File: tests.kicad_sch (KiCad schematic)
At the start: 11 parts, among them J101 USB_A+C+XT30

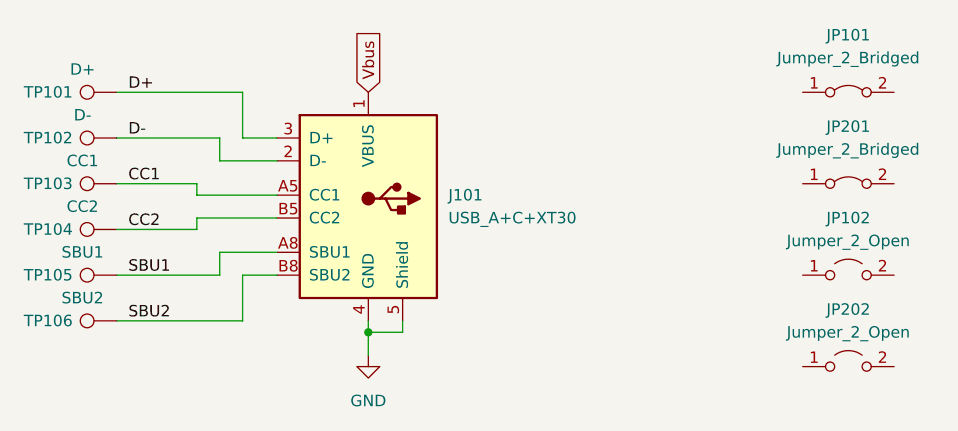
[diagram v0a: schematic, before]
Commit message: ...
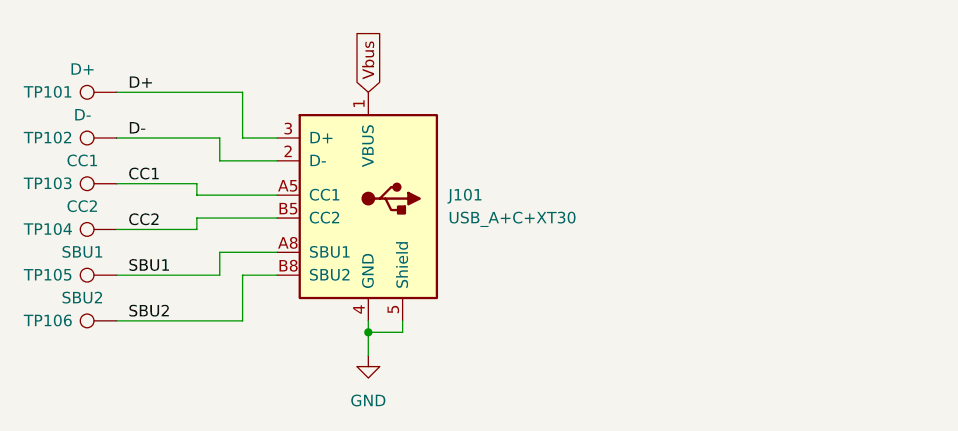
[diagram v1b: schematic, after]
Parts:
- removed JP101: Jumper_2_Bridged, Customs:tinySJ-Bridged, symbol Jumper:Jumper_2_Bridged
- removed JP102: Jumper_2_Open, Customs:tinySJ-Open, symbol Jumper:Jumper_2_Open
- removed JP201: Jumper_2_Bridged, Jumper:SolderJumper-2_P1.3mm_Bridged_RoundedPad1.0x1.5mm, symbol Jumper:Jumper_2_Bridged
- removed JP202: Jumper_2_Open, Jumper:SolderJumper-2_P1.3mm_Open_RoundedPad1.0x1.5mm, symbol Jumper:Jumper_2_Open
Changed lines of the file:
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@@
     )
-  )
-  (symbol (lib_id "Jumper:Jumper_2_Open") (at 194.31 118.11 0) (unit 1)
-    (in_bom yes) (on_board yes) (fields_autoplaced)
-    (property "Reference" "JP202" (id 0) (at 194.31 111.76 0))
-    (property "Value" "Jumper_2_Open" (id 1) (at 194.31 114.3 0))
-    (property "Footprint" "Jumper:SolderJumper-2_P1.3mm_Open_RoundedPad1.0x1.5mm" (id 2) (at 194.31 118.11 0)
-      (effects (font (size 1.27 1.27)) hide)
-    )
-    (property "Datasheet" "~" (id 3) (at 194.31 118.11 0)
-      (effects (font (size 1.27 1.27)) hide)
-    )
-    (pin "1")
-    (pin "2")
   )
   (symbol (lib_id "Connector:TestPoint") (at 113.03 97.79 90) (unit 1)
@@
     )
     (pin "1")
-  )
-  (symbol (lib_id "Jumper:Jumper_2_Bridged") (at 194.31 87.63 0) (unit 1)
-    (in_bom yes) (on_board yes) (fields_autoplaced)
-    (property "Reference" "JP101" (id 0) (at 194.31 81.28 0))
-    (property "Value" "Jumper_2_Bridged" (id 1) (at 194.31 83.82 0))
-    (property "Footprint" "Customs:tinySJ-Bridged" (id 2) (at 194.31 87.63 0)
-      (effects (font (size 1.27 1.27)) hide)
-    )
-    (property "Datasheet" "~" (id 3) (at 194.31 87.63 0)
-      (effects (font (size 1.27 1.27)) hide)
-    )
-    (pin "1")
-    (pin "2")
-  )
-  (symbol (lib_id "Jumper:Jumper_2_Open") (at 194.31 107.95 0) (unit 1)
-    (in_bom yes) (on_board yes) (fields_autoplaced)
-    (property "Reference" "JP102" (id 0) (at 194.31 101.6 0))
-    (property "Value" "Jumper_2_Open" (id 1) (at 194.31 104.14 0))
-    (property "Footprint" "Customs:tinySJ-Open" (id 2) (at 194.31 107.95 0)
-      (effects (font (size 1.27 1.27)) hide)
-    )
-    (property "Datasheet" "~" (id 3) (at 194.31 107.95 0)
-      (effects (font (size 1.27 1.27)) hide)
-    )
-    (pin "1")
-    (pin "2")
-  )
-  (symbol (lib_id "Jumper:Jumper_2_Bridged") (at 194.31 97.79 0) (unit 1)
-    (in_bom yes) (on_board yes) (fields_autoplaced)
-    (property "Reference" "JP201" (id 0) (at 194.31 91.44 0))
-    (property "Value" "Jumper_2_Bridged" (id 1) (at 194.31 93.98 0))
-    (property "Footprint" "Jumper:SolderJumper-2_P1.3mm_Bridged_RoundedPad1.0x1.5mm" (id 2) (at 194.31 97.79 0)
-      (effects (font (size 1.27 1.27)) hide)
-    )
-    (property "Datasheet" "~" (id 3) (at 194.31 97.79 0)
-      (effects (font (size 1.27 1.27)) hide)
-    )
-    (pin "1")
-    (pin "2")
   )
   (symbol (lib_id "USB_A-C_2.0_XT30:USB_A+C+XT30") (at 140.97 100.33 0) (unit 1)
@@
       (reference "J101") (unit 1) (value "USB_A+C+XT30") (footprint "Customs:USB_A+C+XT30")
     )
-    (path "/5c829c2f-59a3-428e-bbbd-c8c45a83afa7"
-      (reference "JP101") (unit 1) (value "Jumper_2_Bridged") (footprint "Customs:tinySJ-Bridged")
-    )
-    (path "/a9587ecc-0119-41d2-8bc7-d0924a78cf2f"
-      (reference "JP102") (unit 1) (value "Jumper_2_Open") (footprint "Customs:tinySJ-Open")
-    )
-    (path "/aab5d863-5e23-4406-a5b2-43b1a050a2b5"
-      (reference "JP201") (unit 1) (value "Jumper_2_Bridged") (footprint "Jumper:SolderJumper-2_P1.3mm_Bridged_RoundedPad1.0x1.5mm")
-    )
-    (path "/1bed38a6-2383-463b-84e4-04849a0939e6"
-      (reference "JP202") (unit 1) (value "Jumper_2_Open") (footprint "Jumper:SolderJumper-2_P1.3mm_Open_RoundedPad1.0x1.5mm")
-    )
     (path "/df616f14-99b7-4644-85ed-e6a688c64b2e"

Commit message: Added tiny Solder Jumpers
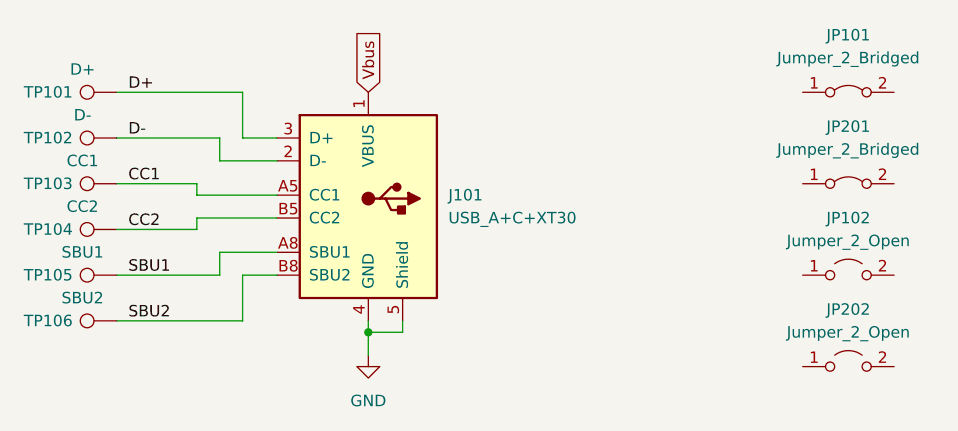
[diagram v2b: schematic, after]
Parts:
- added JP101: Jumper_2_Bridged, Customs:tinySJ-Bridged, symbol Jumper:Jumper_2_Bridged
- added JP102: Jumper_2_Open, Customs:tinySJ-Open, symbol Jumper:Jumper_2_Open
- added JP201: Jumper_2_Bridged, Jumper:SolderJumper-2_P1.3mm_Bridged_RoundedPad1.0x1.5mm, symbol Jumper:Jumper_2_Bridged
- added JP202: Jumper_2_Open, Jumper:SolderJumper-2_P1.3mm_Open_RoundedPad1.0x1.5mm, symbol Jumper:Jumper_2_Open
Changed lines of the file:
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@@
     )
+  )
+  (symbol (lib_id "Jumper:Jumper_2_Open") (at 194.31 118.11 0) (unit 1)
+    (in_bom yes) (on_board yes) (fields_autoplaced)
+    (property "Reference" "JP202" (id 0) (at 194.31 111.76 0))
+    (property "Value" "Jumper_2_Open" (id 1) (at 194.31 114.3 0))
+    (property "Footprint" "Jumper:SolderJumper-2_P1.3mm_Open_RoundedPad1.0x1.5mm" (id 2) (at 194.31 118.11 0)
+      (effects (font (size 1.27 1.27)) hide)
+    )
+    (property "Datasheet" "~" (id 3) (at 194.31 118.11 0)
+      (effects (font (size 1.27 1.27)) hide)
+    )
+    (pin "1")
+    (pin "2")
   )
   (symbol (lib_id "Connector:TestPoint") (at 113.03 97.79 90) (unit 1)
@@
     )
     (pin "1")
+  )
+  (symbol (lib_id "Jumper:Jumper_2_Bridged") (at 194.31 87.63 0) (unit 1)
+    (in_bom yes) (on_board yes) (fields_autoplaced)
+    (property "Reference" "JP101" (id 0) (at 194.31 81.28 0))
+    (property "Value" "Jumper_2_Bridged" (id 1) (at 194.31 83.82 0))
+    (property "Footprint" "Customs:tinySJ-Bridged" (id 2) (at 194.31 87.63 0)
+      (effects (font (size 1.27 1.27)) hide)
+    )
+    (property "Datasheet" "~" (id 3) (at 194.31 87.63 0)
+      (effects (font (size 1.27 1.27)) hide)
+    )
+    (pin "1")
+    (pin "2")
+  )
+  (symbol (lib_id "Jumper:Jumper_2_Open") (at 194.31 107.95 0) (unit 1)
+    (in_bom yes) (on_board yes) (fields_autoplaced)
+    (property "Reference" "JP102" (id 0) (at 194.31 101.6 0))
+    (property "Value" "Jumper_2_Open" (id 1) (at 194.31 104.14 0))
+    (property "Footprint" "Customs:tinySJ-Open" (id 2) (at 194.31 107.95 0)
+      (effects (font (size 1.27 1.27)) hide)
+    )
+    (property "Datasheet" "~" (id 3) (at 194.31 107.95 0)
+      (effects (font (size 1.27 1.27)) hide)
+    )
+    (pin "1")
+    (pin "2")
+  )
+  (symbol (lib_id "Jumper:Jumper_2_Bridged") (at 194.31 97.79 0) (unit 1)
+    (in_bom yes) (on_board yes) (fields_autoplaced)
+    (property "Reference" "JP201" (id 0) (at 194.31 91.44 0))
+    (property "Value" "Jumper_2_Bridged" (id 1) (at 194.31 93.98 0))
+    (property "Footprint" "Jumper:SolderJumper-2_P1.3mm_Bridged_RoundedPad1.0x1.5mm" (id 2) (at 194.31 97.79 0)
+      (effects (font (size 1.27 1.27)) hide)
+    )
+    (property "Datasheet" "~" (id 3) (at 194.31 97.79 0)
+      (effects (font (size 1.27 1.27)) hide)
+    )
+    (pin "1")
+    (pin "2")
   )
   (symbol (lib_id "USB_A-C_2.0_XT30:USB_A+C+XT30") (at 140.97 100.33 0) (unit 1)
@@
       (reference "J101") (unit 1) (value "USB_A+C+XT30") (footprint "Customs:USB_A+C+XT30")
     )
+    (path "/5c829c2f-59a3-428e-bbbd-c8c45a83afa7"
+      (reference "JP101") (unit 1) (value "Jumper_2_Bridged") (footprint "Customs:tinySJ-Bridged")
+    )
+    (path "/a9587ecc-0119-41d2-8bc7-d0924a78cf2f"
+      (reference "JP102") (unit 1) (value "Jumper_2_Open") (footprint "Customs:tinySJ-Open")
+    )
+    (path "/aab5d863-5e23-4406-a5b2-43b1a050a2b5"
+      (reference "JP201") (unit 1) (value "Jumper_2_Bridged") (footprint "Jumper:SolderJumper-2_P1.3mm_Bridged_RoundedPad1.0x1.5mm")
+    )
+    (path "/1bed38a6-2383-463b-84e4-04849a0939e6"
+      (reference "JP202") (unit 1) (value "Jumper_2_Open") (footprint "Jumper:SolderJumper-2_P1.3mm_Open_RoundedPad1.0x1.5mm")
+    )
     (path "/df616f14-99b7-4644-85ed-e6a688c64b2e"
